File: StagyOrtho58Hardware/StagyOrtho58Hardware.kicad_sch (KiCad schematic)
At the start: 73 parts, among them J11 USB_C_Receptacle, SW11 SW_Push, SW12 SW_Push, SW13 SW_Push, SW14 SW_Push, SW15 SW_Push, SW16 SW_Push, SW17 SW_Push, SW18 SW_Push, SW19 SW_Push, SW20 SW_Push, SW21 SW_Push, SW22 SW_Push, SW23 SW_Push, SW24 SW_Push, SW25 SW_Push, SW26 SW_Push, SW27 SW_Push, SW28 SW_Push, SW29 SW_Push, SW30 SW_Push, SW31 SW_Push, SW32 SW_Push, SW33 SW_Push, SW34 SW_Push, SW35 SW_Push, SW36 SW_Push, SW37 SW_Push, SW38 SW_Push, SW39 SW_Push, SW40 SW_Push, U11 Pico, U12 MCP23S17_ML

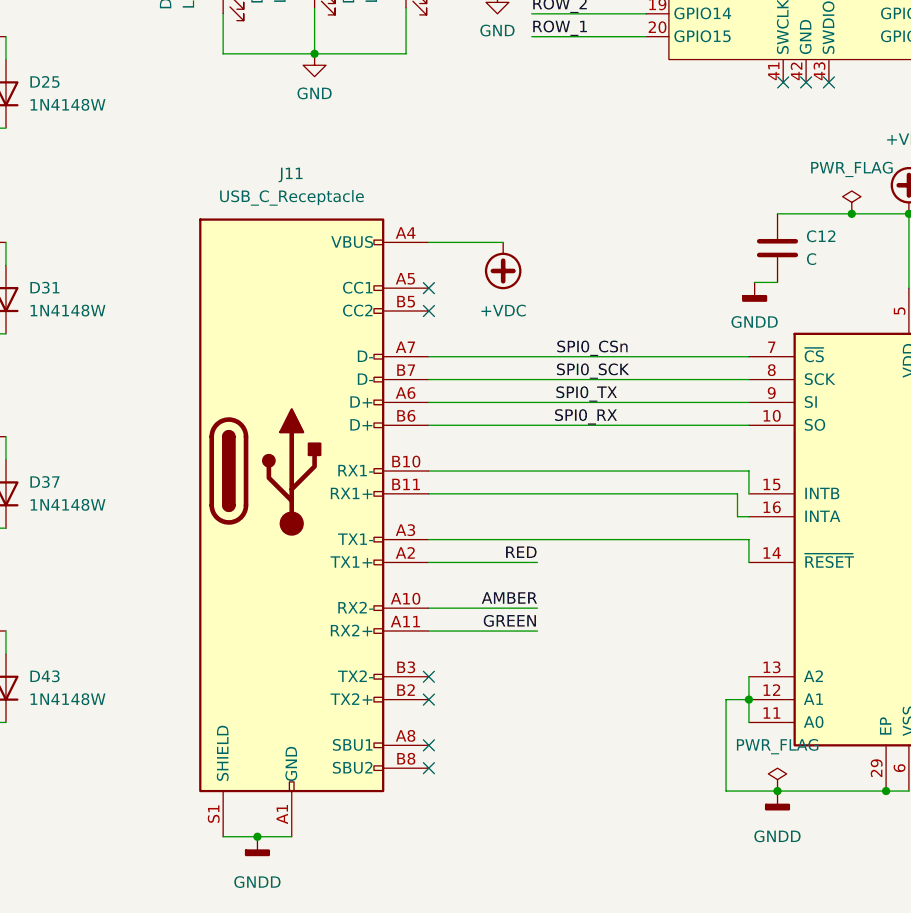
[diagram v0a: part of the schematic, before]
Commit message: Comfortable positions of the keys, ready to layout
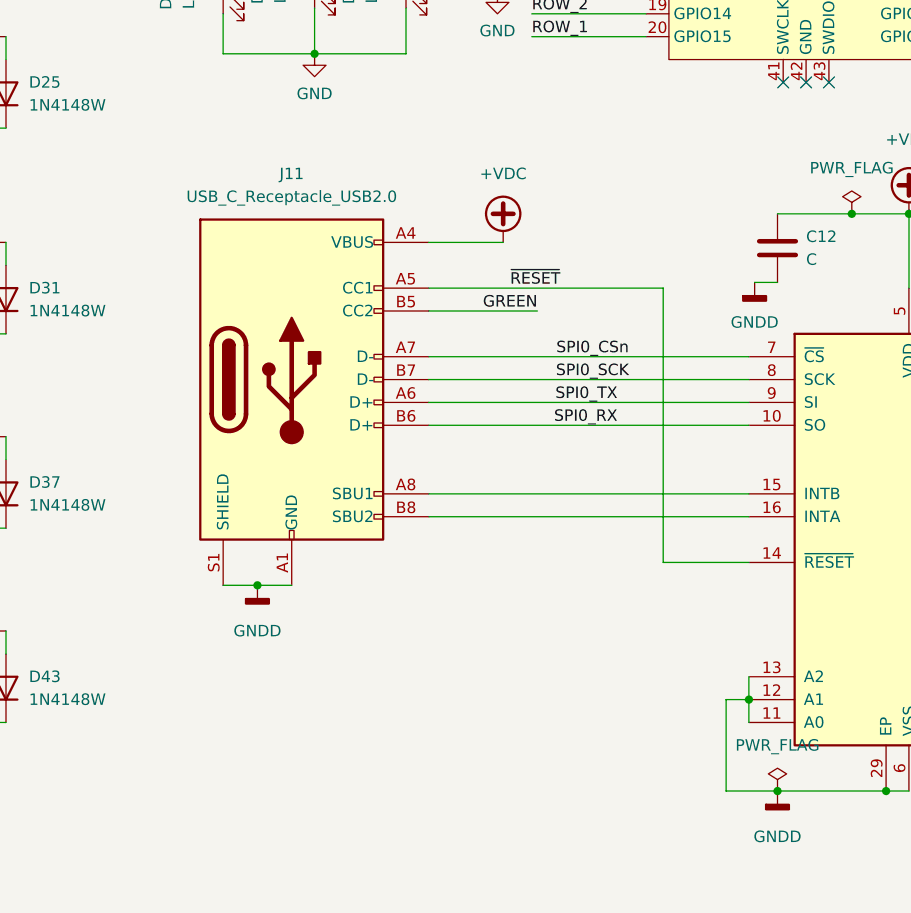
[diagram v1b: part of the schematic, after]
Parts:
- removed J11: USB_C_Receptacle, Connector_USB:USB_C_Receptacle_GCT_USB4085, symbol Connector:USB_C_Receptacle
- added J11: USB_C_Receptacle_USB2.0, Connector_USB:USB_C_Receptacle_GCT_USB4085, symbol Connector:USB_C_Receptacle_USB2.0
- SW29: footprint Switch_Keyboard_Kailh:SW_Kailh_Choc_V1V2_1.50u -> Switch_Keyboard_Kailh:SW_Kailh_Choc_V1V2_2.00u
- SW35, SW37: footprint Switch_Keyboard_Kailh:SW_Kailh_Choc_V1V2_1.50u -> Switch_Keyboard_Kailh:SW_Kailh_Choc_V1V2_1.00u
- SW38: footprint Switch_Keyboard_Kailh:SW_Kailh_Choc_V1V2_1.50u_90deg -> Switch_Keyboard_Kailh:SW_Kailh_Choc_V1V2_1.00u
- SW39: footprint Switch_Keyboard_Kailh:SW_Kailh_Choc_V1V2_2.00u -> Switch_Keyboard_Kailh:SW_Kailh_Choc_V1V2_1.00u
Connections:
- net +VDC: now also J11.A4 (VBUS), J11.A9 (VBUS), J11.B4 (VBUS), J11.B9 (VBUS)
- net GNDD: now also J11.A1 (GND), J11.A12 (GND), J11.B1 (GND), J11.B12 (GND), J11.S1 (SHIELD)
- net GREEN: now also J11.B5 (CC2)
- net SPI0_CSn: now also J11.A7 (D-)
- net SPI0_RX: now also J11.B6 (D+)
- net SPI0_SCK: now also J11.B7 (D-)
- net SPI0_TX: now also J11.A6 (D+)
- net ~{RESET}: now reaches U12.14 (~{RESET})
- net ~{RESET}: now also J11.A5 (CC1)
- net at U12.15 (INTB): now also J11.A8 (SBU1)
- net at U12.16 (INTA): now also J11.B8 (SBU2)
- no-connect marks 28 -> 22
